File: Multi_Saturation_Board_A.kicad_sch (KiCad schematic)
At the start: 46 parts, among them J6 EURO_PWR_2x5, J7 EuroPower_JST_3P, J8 Board_A_1, J9 Board_A_2, U1 NE5532, U2 NE5532, U3 VTL5C, U4 NE5532, U5 NE5532

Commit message: All boards routed
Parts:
- C4, C5: footprint DIYSynthMNL:CP_Radial_D4.0mm_P1.50mm -> Capacitor_THT:CP_Radial_D5.0mm_P2.50mm
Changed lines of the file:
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@@
       (effects (font (size 1.27 1.27)) (justify left))
     )
-    (property "Footprint" "DIYSynthMNL:CP_Radial_D4.0mm_P1.50mm" (at 86.6902 186.055 0)
+    (property "Footprint" "Capacitor_THT:CP_Radial_D5.0mm_P2.50mm" (at 86.6902 186.055 0)
       (effects (font (size 1.27 1.27)) hide)
     )
@@
       (effects (font (size 1.27 1.27)) (justify left))
     )
-    (property "Footprint" "DIYSynthMNL:CP_Radial_D4.0mm_P1.50mm" (at 86.6902 178.435 0)
-      (effects (font (size 1.27 1.27)) hide)
-    )
+    (property "Footprint" "Capacitor_THT:CP_Radial_D5.0mm_P2.50mm" (at 86.6902 178.435 0)
+      (effects (font (size 1.27 1.27)) hide)
+    )

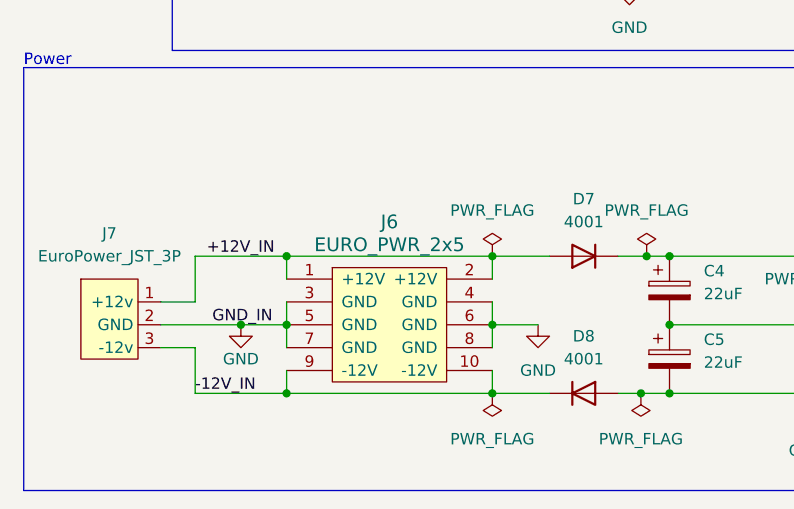
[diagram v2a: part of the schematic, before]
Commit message: board update
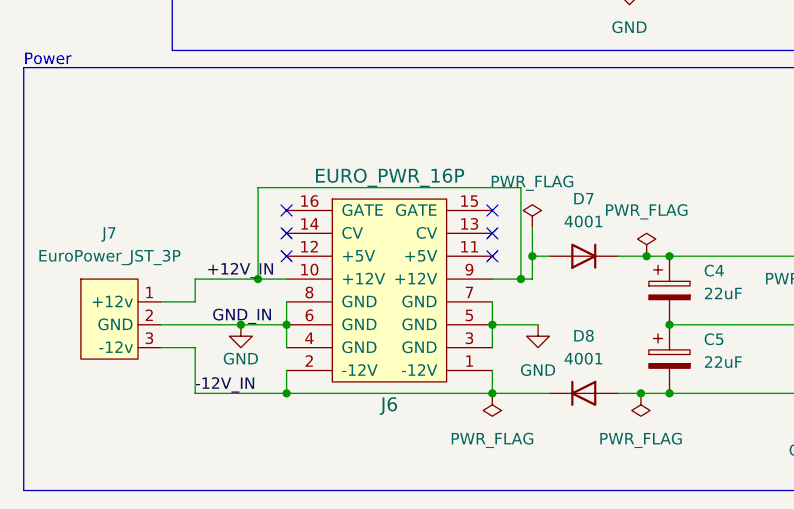
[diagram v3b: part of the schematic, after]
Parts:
- J6: value EURO_PWR_2x5 -> EURO_PWR_16P; footprint DIYSynthMNL:IDC-Header_2x05_P2.54mm_Vertical_BigPads -> DIYSynthMNL:IDC-Header_2x08_P2.54mm_Vertical; symbol eurocad:EURO_PWR_2x5 -> DIYSynthMNL:EURO_PWR_16_PIN
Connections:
- net +12V_IN: now also J6.10 (+12V), J6.9 (+12V); no longer J6.1 (+12V), J6.2 (+12V)
- net -12V_IN: now also J6.1 (-12V), J6.2 (-12V); no longer J6.10 (-12V), J6.9 (-12V)
- no-connect marks 3 -> 9
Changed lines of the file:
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@@
   (junction (at 231.14 59.055) (diameter 0) (color 0 0 0 0)
   )
+  (junction (at 70.485 170.815) (diameter 0) (color 0 0 0 0)
+  )
   (junction (at 241.3 59.055) (diameter 0) (color 0 0 0 0)
   )
@@
   (junction (at 81.28 116.205) (diameter 0) (color 0 0 0 0)
   )
+  (junction (at 40.005 173.355) (diameter 0) (color 0 0 0 0)
+  )
   (junction (at 151.765 165.735) (diameter 0) (color 0 0 0 0)
   )
@@
   (junction (at 121.285 170.815) (diameter 0) (color 0 0 0 0)
   )
-  (junction (at 66.04 170.815) (diameter 0) (color 0 0 0 0)
-  )
   (junction (at 83.185 170.815) (diameter 0) (color 0 0 0 0)
   )
   (junction (at 82.55 186.055) (diameter 0) (color 0 0 0 0)
   )
+  (junction (at 69.215 173.355) (diameter 0) (color 0 0 0 0)
+  )
   (junction (at 131.445 170.815) (diameter 0) (color 0 0 0 0)
   )
   (junction (at 137.16 111.125) (diameter 0) (color 0 0 0 0)
   )
-  (junction (at 43.18 170.815) (diameter 0) (color 0 0 0 0)
-  )
   (junction (at 234.95 85.725) (diameter 0) (color 0 0 0 0)
   )
@@
   )
   (no_connect (at 203.2 126.365))
+  (no_connect (at 66.04 165.735))
+  (no_connect (at 43.18 170.815))
   (no_connect (at 93.98 42.545))
+  (no_connect (at 43.18 168.275))
+  (no_connect (at 66.04 168.275))
   (no_connect (at 104.14 42.545))
+  (no_connect (at 66.04 170.815))
+  (no_connect (at 43.18 165.735))
   (wire (pts (xy 231.14 62.865) (xy 231.14 59.055))
     (stroke (width 0) (type default))
@@
     (stroke (width 0) (type default))
   )
+  (wire (pts (xy 66.04 173.355) (xy 69.215 173.355))
+    (stroke (width 0) (type default))
+  )
   (wire (pts (xy 137.16 111.125) (xy 140.97 111.125))
     (stroke (width 0) (type default))
@@
     (stroke (width 0) (type default))
   )
+  (wire (pts (xy 70.485 170.815) (xy 70.485 173.355))
+    (stroke (width 0) (type default))
+  )
   (wire (pts (xy 158.75 41.275) (xy 158.75 48.895))
     (stroke (width 0) (type default))
@@
     (stroke (width 0) (type default))
   )
+  (wire (pts (xy 69.215 163.195) (xy 69.215 173.355))
+    (stroke (width 0) (type default))
+  )
   (wire (pts (xy 44.45 42.545) (xy 43.18 42.545))
     (stroke (width 0) (type default))
@@
     (stroke (width 0) (type default))
   )
-  (wire (pts (xy 66.04 170.815) (xy 43.18 170.815))
+  (wire (pts (xy 229.235 146.685) (xy 229.235 149.225))
     (stroke (width 0) (type default))
   )
-  (wire (pts (xy 229.235 146.685) (xy 229.235 149.225))
+  (wire (pts (xy 69.215 173.355) (xy 70.485 173.355))
     (stroke (width 0) (type default))
   )
@@
     (stroke (width 0) (type default))
   )
+  (wire (pts (xy 70.485 170.815) (xy 72.39 170.815))
+    (stroke (width 0) (type default))
+  )
+  (wire (pts (xy 40.005 163.195) (xy 69.215 163.195))
+    (stroke (width 0) (type default))
+  )
   (wire (pts (xy 85.725 170.815) (xy 111.125 170.815))
     (stroke (width 0) (type default))
@@
     (stroke (width 0) (type default))
   )
-  (wire (pts (xy 66.04 170.815) (xy 72.39 170.815))
-    (stroke (width 0) (type default))
-  )
   (wire (pts (xy 113.03 186.055) (xy 113.03 189.865))
     (stroke (width 0) (type default))
@@
     (stroke (width 0) (type default))
   )
-  (wire (pts (xy 33.02 175.895) (xy 33.02 170.815))
+  (wire (pts (xy 33.02 175.895) (xy 33.02 173.355))
     (stroke (width 0) (type default))
   )
@@
     (stroke (width 0) (type default))
   )
-  (wire (pts (xy 66.04 173.355) (xy 66.04 170.815))
-    (stroke (width 0) (type default))
-  )
   (wire (pts (xy 219.71 61.595) (xy 219.71 59.055))
     (stroke (width 0) (type default))
@@
     (stroke (width 0) (type default))
   )
+  (wire (pts (xy 33.02 173.355) (xy 40.005 173.355))
+    (stroke (width 0) (type default))
+  )
   (wire (pts (xy 137.16 111.125) (xy 137.16 115.57))
     (stroke (width 0) (type default))
@@
     (stroke (width 0) (type default))
   )
-  (wire (pts (xy 43.18 170.815) (xy 43.18 173.355))
-    (stroke (width 0) (type default))
-  )
   (wire (pts (xy 203.2 118.745) (xy 203.2 121.285))
     (stroke (width 0) (type default))
@@
     (stroke (width 0) (type default))
   )
+  (wire (pts (xy 40.005 173.355) (xy 43.18 173.355))
+    (stroke (width 0) (type default))
+  )
   (wire (pts (xy 139.7 38.735) (xy 143.51 38.735))
     (stroke (width 0) (type default))
   )
+  (wire (pts (xy 70.485 167.64) (xy 70.485 170.815))
+    (stroke (width 0) (type default))
+  )
   (wire (pts (xy 189.23 56.515) (xy 204.47 56.515))
     (stroke (width 0) (type default))
@@
     (stroke (width 0) (type default))
   )
-  (wire (pts (xy 33.02 170.815) (xy 43.18 170.815))
+  (wire (pts (xy 40.005 173.355) (xy 40.005 163.195))
     (stroke (width 0) (type default))
   )
@@
     (effects (font (size 1.27 1.27)) (justify left bottom))
   )
-  (label "+12V_IN" (at 34.29 170.815 0) (fields_autoplaced)
+  (label "+12V_IN" (at 34.29 173.355 0) (fields_autoplaced)
     (effects (font (size 1.27 1.27)) (justify left bottom))
   )
@@
     )
   )
-  (symbol (lib_id "power:PWR_FLAG") (at 66.04 170.815 0) (unit 1)
+  (symbol (lib_id "power:PWR_FLAG") (at 70.485 167.64 0) (unit 1)
     (in_bom yes) (on_board yes) (dnp no)
-    (property "Reference" "#FLG?" (at 66.04 168.91 0)
+    (property "Reference" "#FLG?" (at 70.485 165.735 0)
       (effects (font (size 1.27 1.27)) hide)
     )
-    (property "Value" "PWR_FLAG" (at 66.04 165.735 0)
+    (property "Value" "PWR_FLAG" (at 70.485 162.56 0)
       (effects (font (size 1.27 1.27)))
     )
-    (property "Footprint" "" (at 66.04 170.815 0)
+    (property "Footprint" "" (at 70.485 167.64 0)
       (effects (font (size 1.27 1.27)) hide)
     )
-    (property "Datasheet" "~" (at 66.04 170.815 0)
+    (property "Datasheet" "~" (at 70.485 167.64 0)
       (effects (font (size 1.27 1.27)) hide)
     )
@@
     )
   )
-  (symbol (lib_id "eurocad:EURO_PWR_2x5") (at 54.61 178.435 0) (unit 1)
+  (symbol (lib_id "DIYSynthMNL:EURO_PWR_16_PIN") (at 54.61 178.435 0) (unit 1)
     (in_bom yes) (on_board yes) (dnp no)
-    (property "Reference" "J6" (at 54.61 167.005 0)
+    (property "Reference" "J6" (at 54.61 187.325 0)
       (effects (font (size 1.524 1.524)))
     )
-    (property "Value" "EURO_PWR_2x5" (at 54.61 169.545 0)
+    (property "Value" "EURO_PWR_16P" (at 54.61 161.925 0)
       (effects (font (size 1.524 1.524)))
     )
-    (property "Footprint" "DIYSynthMNL:IDC-Header_2x05_P2.54mm_Vertical_BigPads" (at 53.34 189.865 0)
+    (property "Footprint" "DIYSynthMNL:IDC-Header_2x08_P2.54mm_Vertical" (at 48.895 192.405 0)
       (effects (font (size 1.524 1.524)) hide)
     )
@@
     (pin "7")
     (pin "9")
+    (pin "13")
+    (pin "16")
+    (pin "11")
+    (pin "12")
+    (pin "15")
+    (pin "14")
     (instances
       (project "Multi saturation module"
